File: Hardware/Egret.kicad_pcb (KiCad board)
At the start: 2 copper layers, 64.6 x 60.3 mm, 60 parts, among them Q1 S8050, Q2 S8050, Q3 AO3415AL, SW1 TD-1106SN-5.0H-160, SW2 TD-1106SN-5.0H-160, U1 WS2812B-B, U10 ST7789_FPC_PAD, U2 AN2051-245_2.4G, U3 ESP32--PICO--D4, U4 MPU6050-YJLTY, U5 AMS1117-3.3, U6 BH1750FVI-TR, U7 CP2102N-A02-GQFN28, U8 FPC-SMD_8P-P0.5, U9 FPC-SMD_8P-P0.5

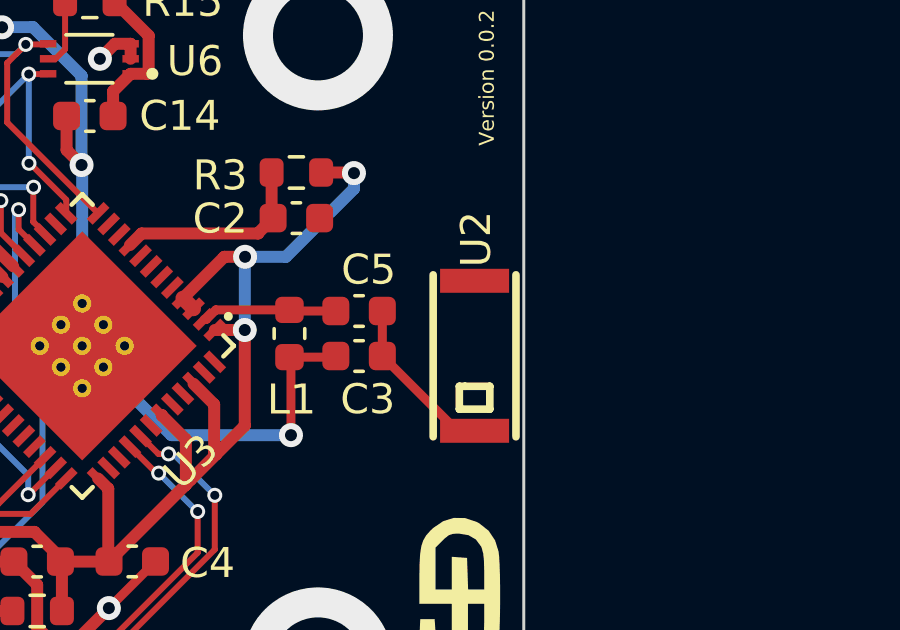
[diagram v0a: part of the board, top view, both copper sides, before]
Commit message: update
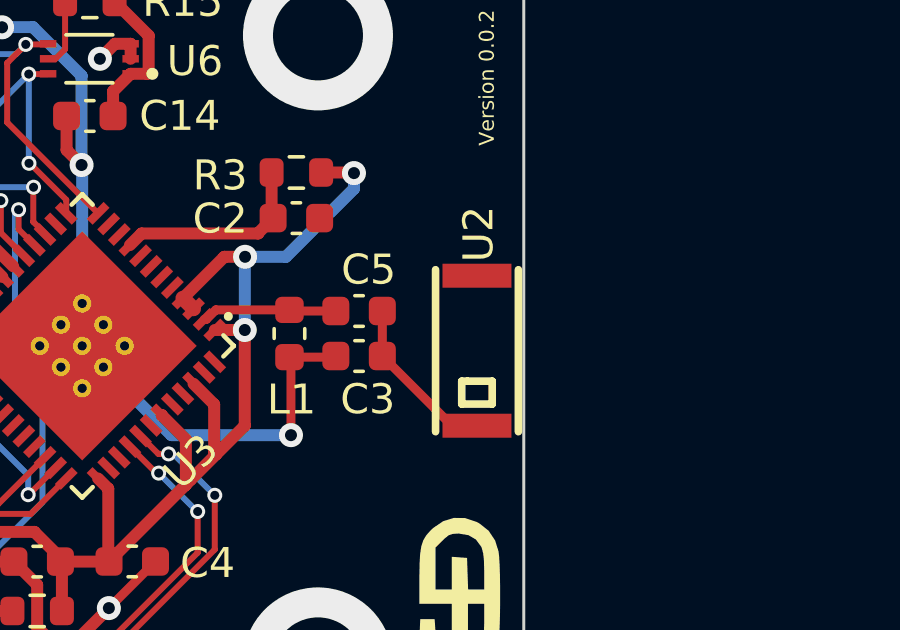
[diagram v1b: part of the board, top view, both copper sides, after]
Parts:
- moved U2 0.19 mm to (179.7, 86.9)
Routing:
- net Net-(C3-Pad1): track 5.02 -> 5.62 mm
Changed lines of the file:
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@@
   )
   (footprint "Uinika.Footprint:ANT-SMD_L5.0-W2.0" (layer "F.Cu")
-    (at 179.62 87.08 90)
+    (at 179.7 86.91 90)
     (property "Sheetfile" "Egret.kicad_sch")
     (property "Sheetname" "")
@@
   (segment (start 168.519233 83.003) (end 168.13099 83.391243) (width 0.4) (layer "F.Cu") (net 3))
   (segment (start 172.407 82.988) (end 172.905 82.49) (width 0.4) (layer "F.Cu") (net 3))
-  (segment (start 176.545 87.0875) (end 179.0375 89.58) (width 0.3) (layer "F.Cu") (net 4))
+  (segment (start 178.8675 89.41) (end 179.7 89.41) (width 0.3) (layer "F.Cu") (net 4))
+  (segment (start 176.545 87.0875) (end 178.8675 89.41) (width 0.3) (layer "F.Cu") (net 4))
   (segment (start 176.545 85.5875) (end 176.545 87.0875) (width 0.3) (layer "F.Cu") (net 4))
   (segment (start 169.19165 89.06165) (end 169.997 89.867) (width 0.4) (layer "F.Cu") (net 5))

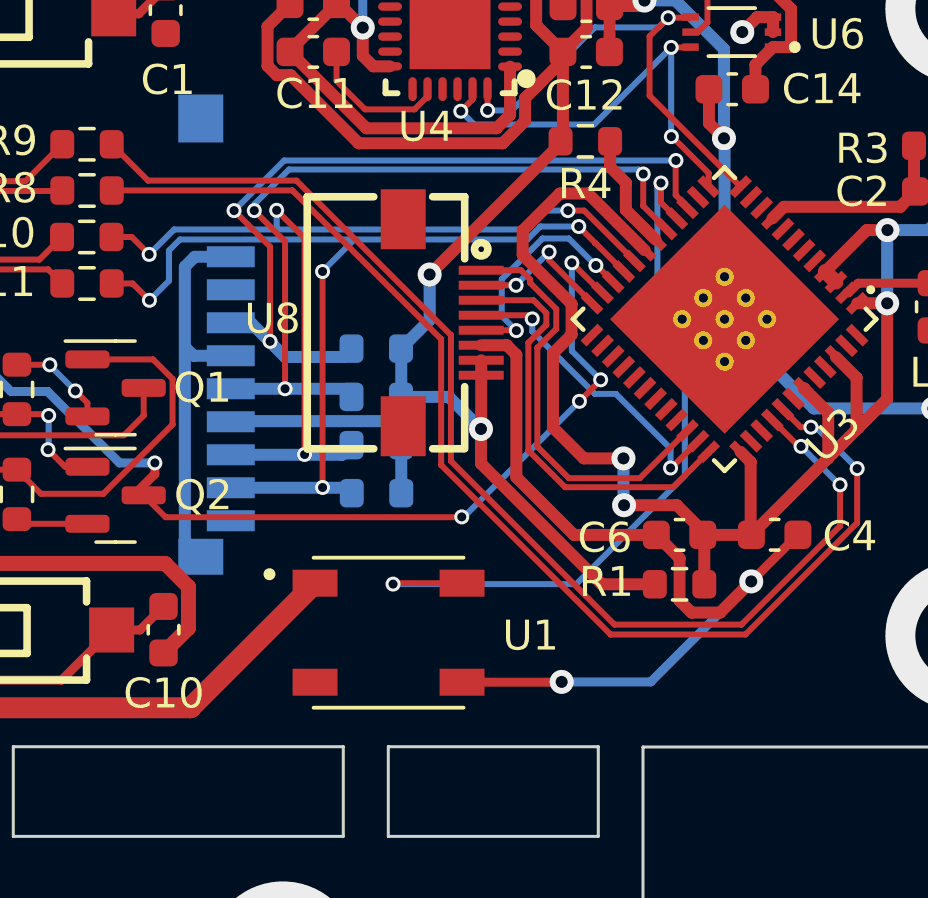
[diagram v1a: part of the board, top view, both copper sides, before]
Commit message: update
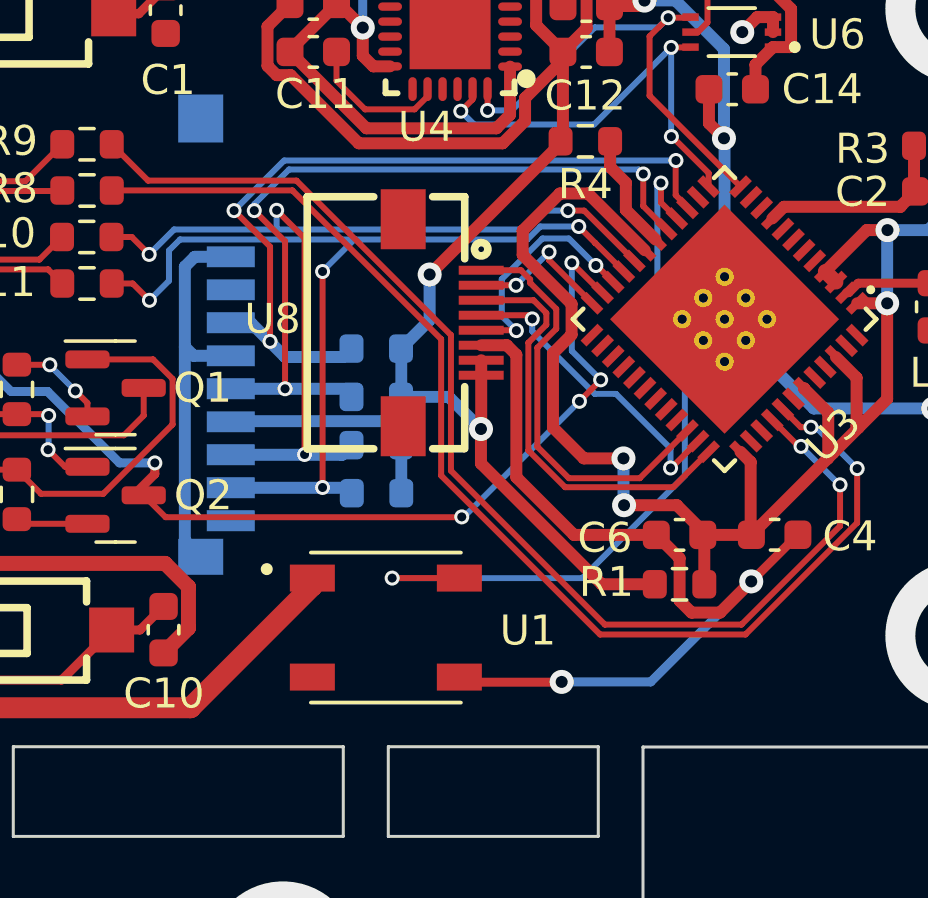
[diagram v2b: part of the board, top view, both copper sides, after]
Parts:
- moved U1 0.19 mm to (155.2, 97.0)
